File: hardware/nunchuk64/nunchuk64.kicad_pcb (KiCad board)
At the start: 2 copper layers, 50 x 41.6 mm, 42 parts, among them J1 DB9_Female, J2 DB9_Female, J3 Conn_02x03_Odd_Even, P1 CONN_WII, P2 CONN_WII, Q1 BSS138, Q2 BSS138, Q3 BSS138, Q4 BSS138, SW1 SW_Push, U1 AMS1117-3V3, U2 ATMEGA328P-AU

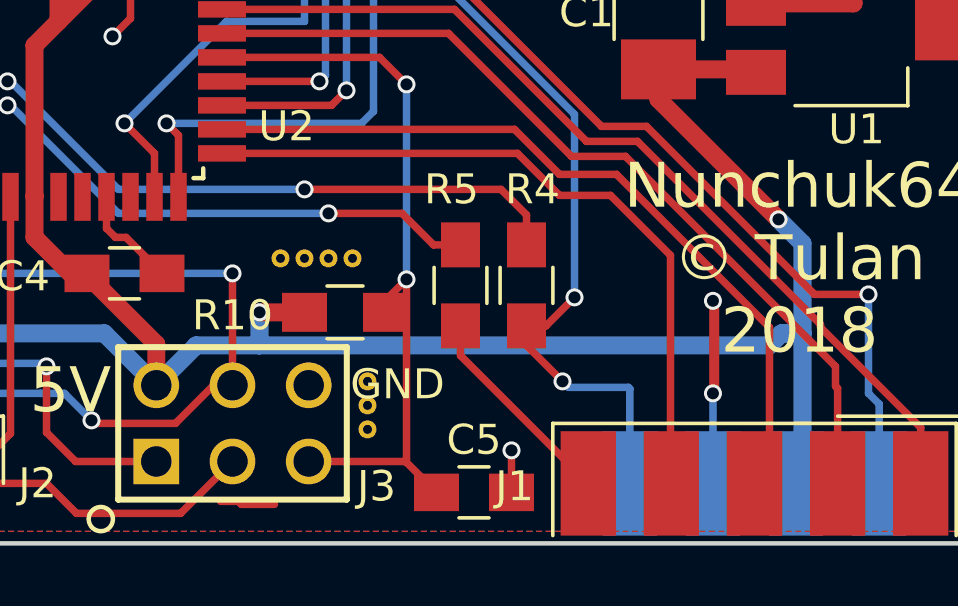
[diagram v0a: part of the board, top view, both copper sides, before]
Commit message: changed layout a bit
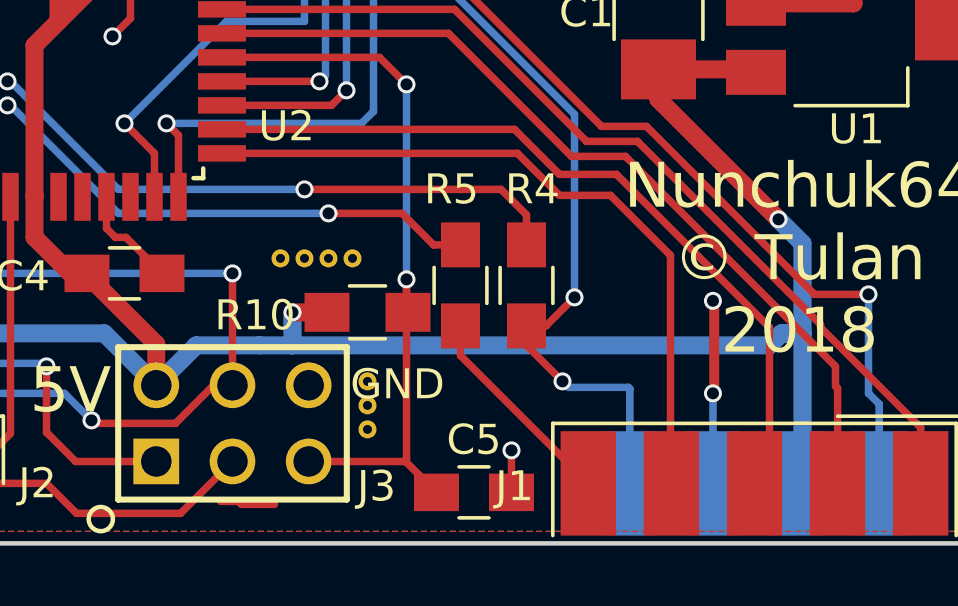
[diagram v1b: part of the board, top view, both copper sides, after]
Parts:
- moved R10 0.75 mm to (104.5, 105.9)
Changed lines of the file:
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@@
   (general
     (links 93)
-    (no_connects 1)
+    (no_connects 0)
     (area 76.324999 71.924999 126.475001 113.675001)
     (thickness 1.6)
     (drawings 12)
-    (tracks 363)
+    (tracks 364)
     (zones 0)
     (modules 42)
@@
   )
   (module Resistors_SMD:R_0805_HandSoldering (layer F.Cu)
-    (at 103.75 105.9)
+    (at 104.5 105.9)
     (descr "Resistor SMD 0805, hand soldering")
     (tags "resistor 0805")
@@
   (segment (start 92.6 94.8) (end 92.6 93.55) (width 0.25) (layer F.Cu) (net 6))
   (via (at 92.6 94.8) (size 0.6) (drill 0.4) (layers F.Cu B.Cu) (net 6))
-  (segment (start 100.9 105.9) (end 102.4 105.9) (width 0.6) (layer F.Cu) (net 7))
+  (segment (start 102 105.9) (end 103.2 105.9) (width 0.6) (layer F.Cu) (net 7))
+  (segment (start 117.9 107) (end 102 107) (width 0.6) (layer B.Cu) (net 7))
+  (segment (start 102 105.9) (end 102 107) (width 0.6) (layer B.Cu) (net 7))
+  (segment (start 102 107) (end 100.9 107) (width 0.6) (layer B.Cu) (net 7))
   (segment (start 100.9 107) (end 98.79 107) (width 0.6) (layer B.Cu) (net 7))
-  (segment (start 117.9 107) (end 100.9 107) (width 0.6) (layer B.Cu) (net 7))
-  (segment (start 100.9 107) (end 100.9 105.9) (width 0.6) (layer B.Cu) (net 7))
-  (via (at 100.9 105.9) (size 0.6) (drill 0.4) (layers F.Cu B.Cu) (net 7))
+  (via (at 102 105.9) (size 0.6) (drill 0.4) (layers F.Cu B.Cu) (net 7))
   (segment (start 118.3 106.6) (end 117.9 107) (width 0.6) (layer B.Cu) (net 7))
   (segment (start 98.79 107) (end 97.46 108.33) (width 0.6) (layer B.Cu) (net 7))
@@
   (segment (start 79.8 102.7) (end 87.5 95) (width 0.25) (layer F.Cu) (net 31))
   (segment (start 87.5 95) (end 91.15 95) (width 0.25) (layer F.Cu) (net 31))
-  (segment (start 105.1 105.9) (end 105.1 105.5) (width 0.25) (layer F.Cu) (net 35))
-  (segment (start 105.1 105.5) (end 105.8 104.8) (width 0.25) (layer F.Cu) (net 35))
+  (segment (start 105.8 104.8) (end 105.8 105.85) (width 0.25) (layer F.Cu) (net 35))
+  (segment (start 105.8 105.85) (end 105.85 105.9) (width 0.25) (layer F.Cu) (net 35))
   (segment (start 105.73 110.87) (end 105.77 110.87) (width 0.25) (layer F.Cu) (net 35))
   (segment (start 105.77 110.87) (end 106.8 111.9) (width 0.25) (layer F.Cu) (net 35))
